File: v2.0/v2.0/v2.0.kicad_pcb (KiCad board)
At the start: 4 copper layers, 84 x 51 mm, 160 parts, among them IC1 STM32N657X0H3Q, J1 Conn_01x05_Pin, J2 Conn_01x02_Pin, U10 XC6206P282MR, U11 XC6206P152MR, U13 48MHz, U4 TPS62088YFP, U8 MX66LM1G45G

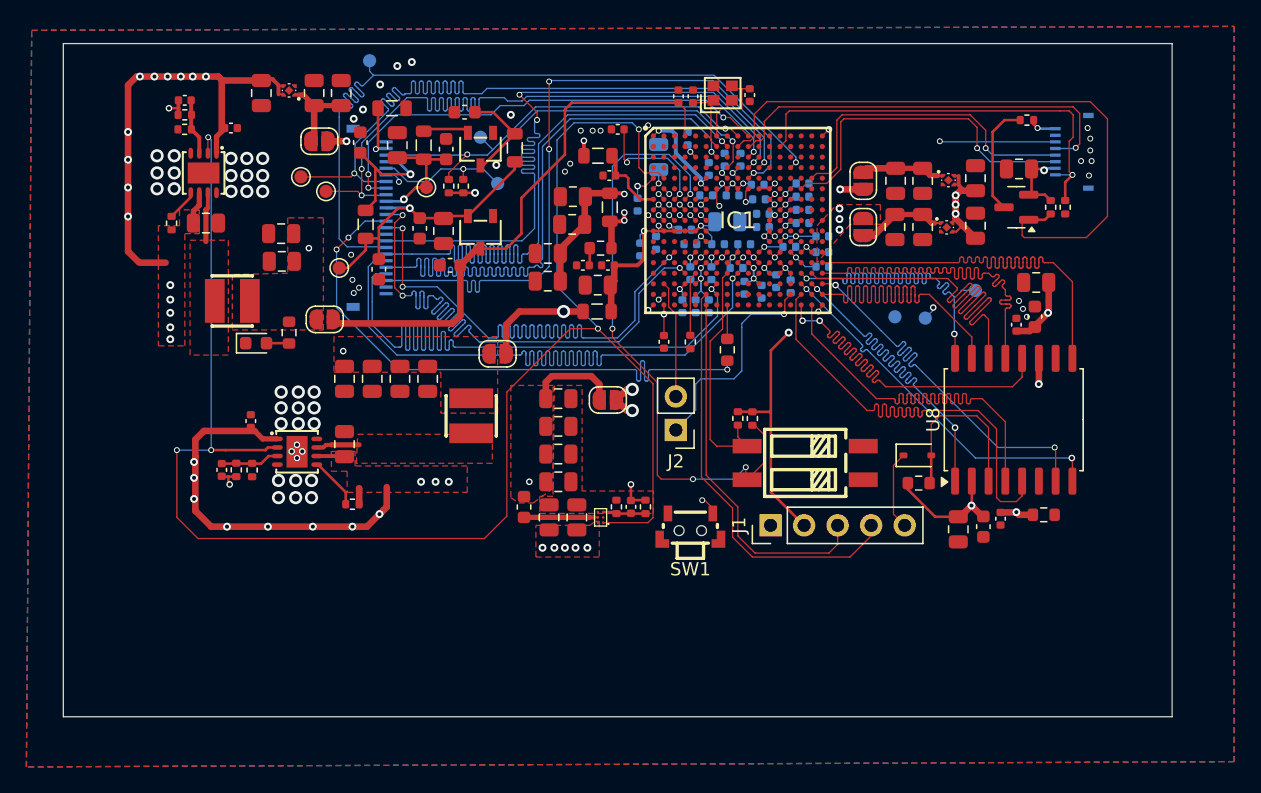
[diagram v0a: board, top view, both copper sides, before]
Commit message: V2.0 Prototype Y61-9265739A
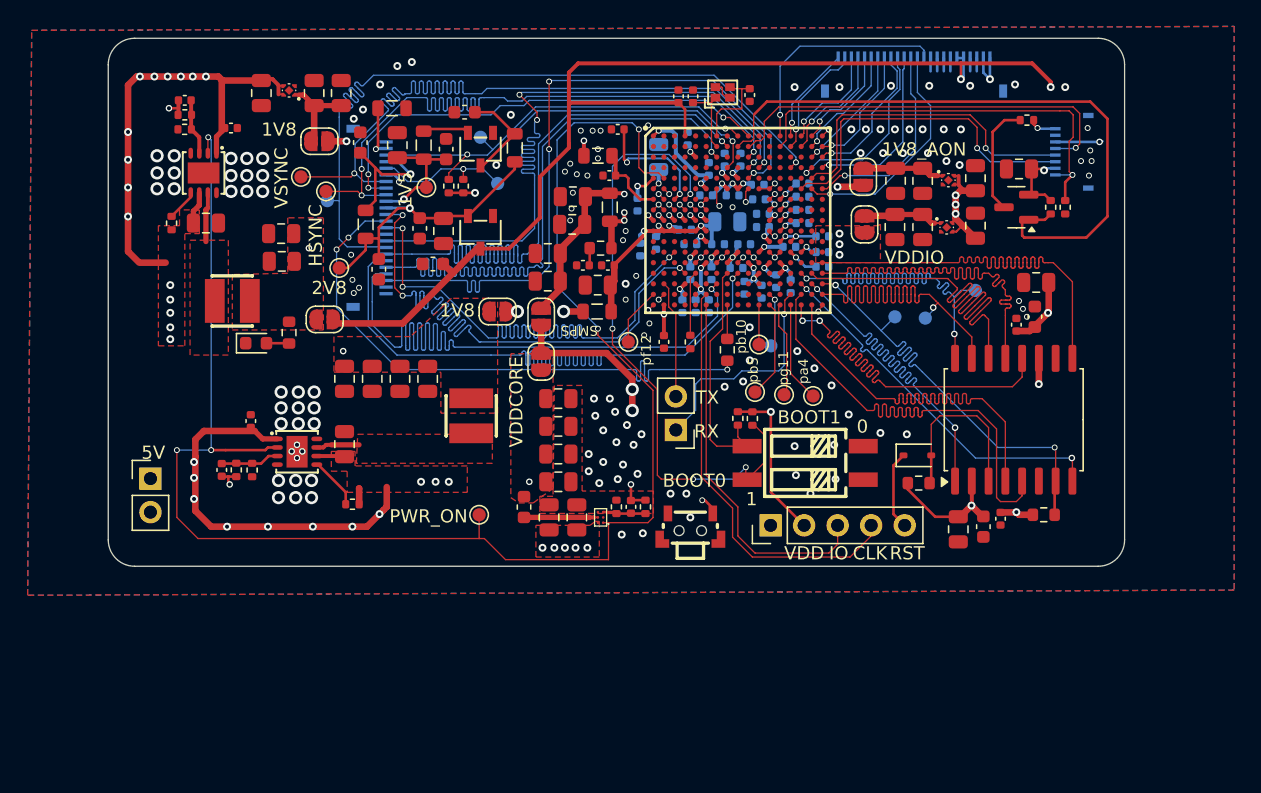
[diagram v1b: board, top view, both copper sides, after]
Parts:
- added J3: Conn_01x02_Pin, Connector_PinHeader_2.54mm:PinHeader_1x02_P2.54mm_Vertical, F.Cu at (89.2, 93.4)
- added JP7: SolderJumper_2_Open, Jumper:SolderJumper-2_P1.3mm_Open_RoundedPad1.0x1.5mm, F.Cu at (118.8, 81.1)
- added TP10: TestPoint, TestPoint:TestPoint_Pad_D1.0mm, F.Cu at (139.4, 87.1)
- added TP11: TestPoint, TestPoint:TestPoint_Pad_D1.0mm, F.Cu at (137.2, 87.0)
- added TP12: TestPoint, TestPoint:TestPoint_Pad_D1.0mm, F.Cu at (135.0, 86.8)
- added TP13: TestPoint, TestPoint:TestPoint_Pad_D1.0mm, F.Cu at (135.3, 83.2)
- added TP14: TestPoint, TestPoint:TestPoint_Pad_D1.0mm, B.Cu at (136.2, 83.3)
- added TP15: TestPoint, TestPoint:TestPoint_Pad_D1.0mm, F.Cu at (125.4, 83.0)
- added TP9: TestPoint, TestPoint:TestPoint_Pad_D1.0mm, F.Cu at (114.1, 96.1)
- added X1: -, v2.0:CRYSTAL-SMD_4P-L1.6-W1.2-BL, F.Cu at (132.6, 64.1)
- U13: value 48MHz -> ~; footprint v2.0:CRYSTAL-SMD_4P-L2.0-W1.6-BL -> Grinreflex:FFC-SMD_24P-P0.50_FH34SRJ-24S-0.5SH; moved to B.Cu
- moved U13 14.6 mm to (147.1, 62.8), turned to 180 degrees
- moved TP6 11.1 mm to (102.6, 72.3)
- moved JP6 5.82 mm to (118.8, 84.5), turned to 90 degrees
- moved JP4 3.20 mm to (115.5, 80.7)
- moved C82 1.30 mm to (110.6, 77.1)
- moved JP1 0.30 mm to (143.2, 70.5)
- moved JP2 0.22 mm to (143.3, 74.1), turned to -90 degrees
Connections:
- C4 pad 2: /VDD_3V3 -> +3V3
- C82 pad 1: /VDD_3V3 -> +3V3
- IC1 pad A13: unconnected-(IC1-PD10-PadA13) -> /MCU/PD10
- IC1 pad A14: unconnected-(IC1-PD1-PadA14) -> /MCU/PD1
- IC1 pad A15: unconnected-(IC1-PE8-PadA15) -> /MCU/PE8
- IC1 pad A16: unconnected-(IC1-PE9-PadA16) -> /MCU/PE9
- IC1 pad A4: /VDD_3V3 -> +3V3
- IC1 pad B14: /MCU/I2C2_SDA -> /MCU/PD15
- IC1 pad B15: unconnected-(IC1-PD4-PadB15) -> /MCU/PD4
- IC1 pad B16: unconnected-(IC1-PE10-PadB16) -> /MCU/PE10
- IC1 pad B17: unconnected-(IC1-PB14-PadB17) -> /MCU/PB14
- IC1 pad C16: unconnected-(IC1-PB2-PadC16) -> /MCU/PB2
- IC1 pad C17: unconnected-(IC1-PD13-PadC17) -> /MCU/PD13
- IC1 pad D16: unconnected-(IC1-PB8-PadD16) -> /MCU/PB8
- IC1 pad D17: unconnected-(IC1-PB15-PadD17) -> /MCU/PB15
- IC1 pad F16: unconnected-(IC1-PE0-PadF16) -> /MCU/PE0
- IC1 pad F17: unconnected-(IC1-PE1-PadF17) -> /MCU/PE1
- IC1 pad T1: unconnected-(IC1-PF12-PadT1) -> Net-(IC1-PF12)
- IC1 pad T12: unconnected-(IC1-PB4-PadT12) -> Net-(IC1-PB4)
- IC1 pad U11: unconnected-(IC1-PB10-PadU11) -> Net-(IC1-PB10)
- IC1 pad U12: unconnected-(IC1-PB5-PadU12) -> Net-(IC1-PB5)
- IC1 pad U13: unconnected-(IC1-PG11-PadU13) -> Net-(IC1-PG11)
- IC1 pad U14: unconnected-(IC1-PA4-PadU14) -> Net-(IC1-PA4)
- JP3 pad 2: /VDD_3V3 -> +3V3
- U10 pad 3: /VDD_3V3 -> +3V3
- U13 pad 1: /MCU/OSC_OUT -> /MCU/PD1
- U13 pad 2: GND -> /MCU/PD15
- U13 pad 3: /MCU/OSC_IN -> /MCU/PE8
- U13 pad 4: GND -> /MCU/PD4
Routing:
- net +3V3: track 5.79 -> 96.1 mm, vias 1 -> 3
- net /VDD_3V3: track 41.3 -> 0.00 mm
- net /VDDIO: track 71.8 -> 95.9 mm, vias 21 -> 22
- net /MCU/PD10: track 0.00 -> 17.5 mm, vias 0 -> 1
- net /MCU/PE0: track 0.00 -> 17.4 mm, vias 0 -> 1
- net /VDDA_1V8: track 66.9 -> 82.8 mm, vias 8 -> 9
- net /MCU/PE1: track 0.00 -> 15.3 mm, vias 0 -> 1
- net /MCU/PB8: track 0.00 -> 14.2 mm, vias 0 -> 1
- net /MCU/PB15: track 0.00 -> 13.3 mm, vias 0 -> 1
- net /RESET: track 169.6 -> 156.8 mm
- net /MCU/PD13: track 0.00 -> 11.1 mm, vias 0 -> 1
- net /MCU/PB2: track 0.00 -> 9.57 mm, vias 0 -> 1
- net /MCU/PB14: track 0.00 -> 9.56 mm, vias 0 -> 1
- net /MCU/PD4: track 0.00 -> 9.07 mm, vias 0 -> 1
- net /MCU/PE10: track 0.00 -> 8.85 mm, vias 0 -> 1
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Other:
- board size 84 x 51 mm -> 77 x 40 mm
- board text added: "0"
- board text added: "1"
- board text added: "100nF"
- board text added: "10uF"
- board text added: "1V5"
- board text added: "1V8"
- board text added: "1V8_AON"
- board text added: "24"
- board text added: "2V8"
- board text added: "5V"
- board text added: "8"
- board text added: "BOOT0"
- board text added: "BOOT1"
- board text added: "CLK"
- board text added: "HSYNC"
- board text added: "IO"
- board text added: "NCS"
- board text added: "PD1 1 PD15 2 PE8 3 PD4 4 PE9 5 PE10 6 PB2 7 PB14 8 PD13 9 PB8 10 PB15 11 PE1 12 PE0 13 PD10 14 GND 15 GND 16 GND 17 GND 18 +3V3 19 +3V3 20 GND 21 GND 22 VDDIO 23 VDDIO 24"
- board text added: "PWR_ON"
- board text added: "RST"
- board text added: "RX"
- board text added: "SCL"
- board text added: "SDA"
- board text added: "SI0"
- board text added: "SMPS"
- board text added: "TX"
- board text added: "VDD"
- board text added: "VDDCORE"
- board text added: "VDDIO"
- board text added: "VSYNC"
- board text added: "pa4"
- board text added: "pb10"
- board text added: "pb4"
- board text added: "pb5"
- board text added: "pf12"
- board text added: "pg11"
